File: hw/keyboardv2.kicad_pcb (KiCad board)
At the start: 2 copper layers, 145 x 45 mm, 40 parts, among them K1 CONN_4, K2 CONN_4, K3 CONN_4, K4 CONN_4, K5 CONN_4, K6 CONN_4, K7 CONN_4, K8 CONN_4, Q1 MOSFET_N, U1 TINYMEGA, U2 74HC595, U3 4051, U4 4051, U5 74HC595

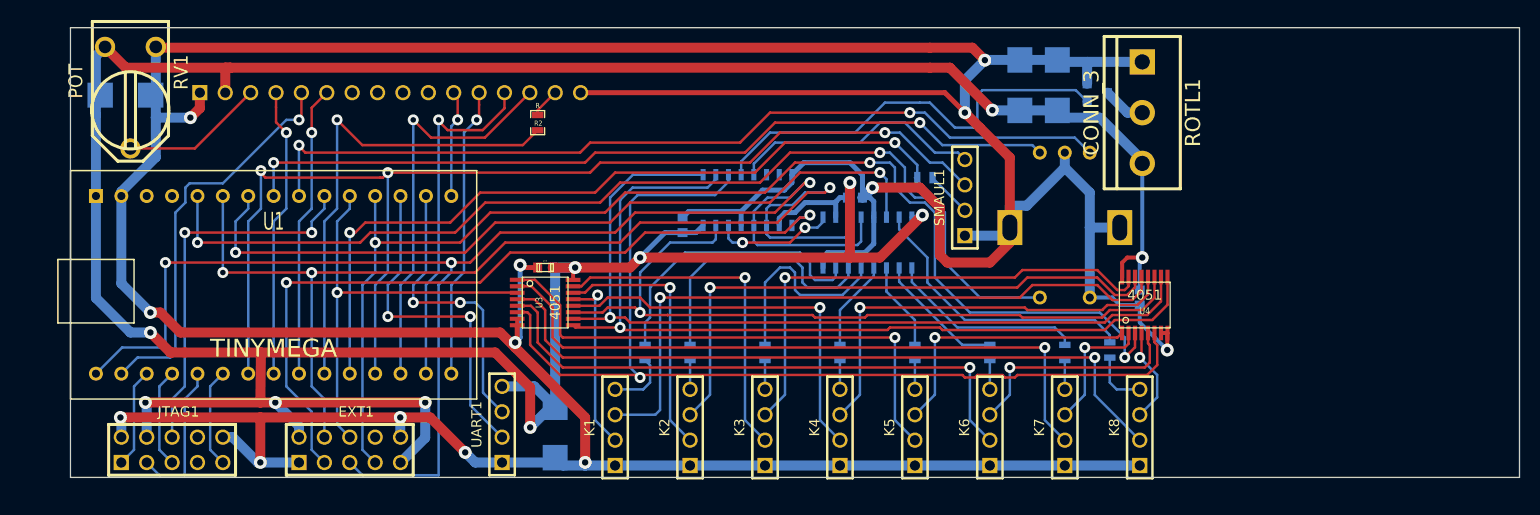
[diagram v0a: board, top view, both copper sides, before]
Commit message: Yeah, so I had the board reversed -.-   Once more with feeling.
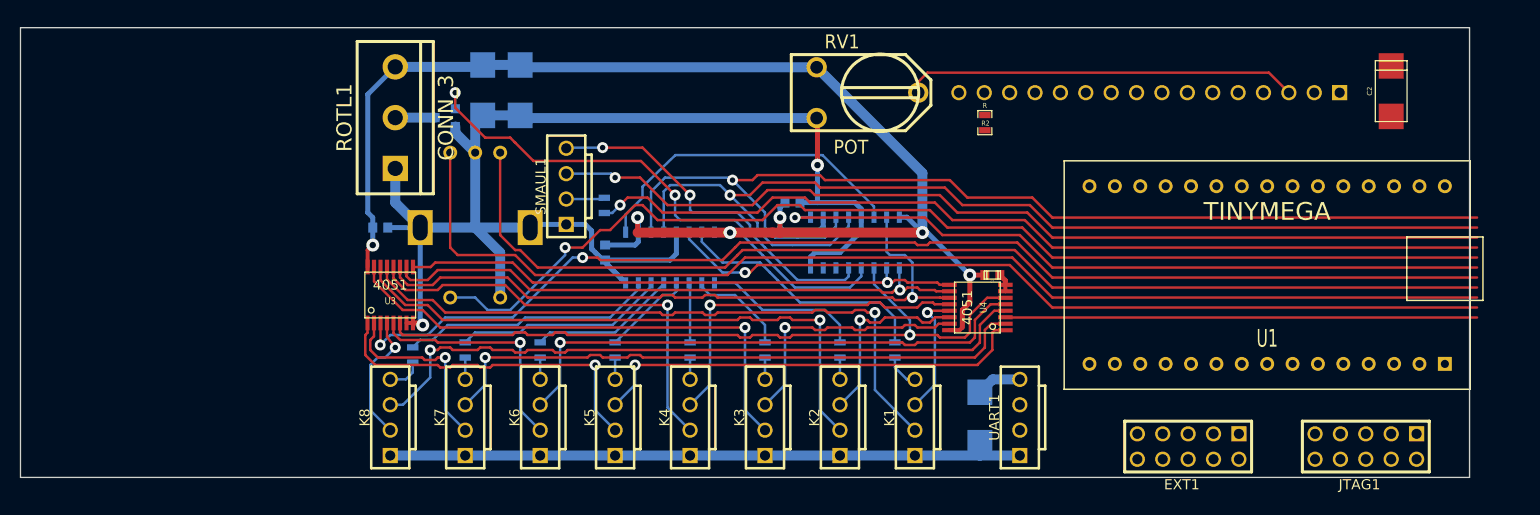
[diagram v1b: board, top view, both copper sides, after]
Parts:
- C2: moved to F.Cu
- K1, K2, K3, K4, K5, K6, K7, K8, SMAUL1, UART1: footprint PIN_ARRAY_4x1_BPAD -> PIN_ARRAY_4x1_KEYED_BPAD
- moved C2 126.7 mm to (212.2, 106.3), turned to 90 degrees
- moved JTAG1 119.5 mm to (209.6, 141.9), turned to 180 degrees
- moved U1 99.4 mm to (199.8, 124.8), turned to 180 degrees
- moved LCD1 95.0 mm to (207.0, 106.5), turned to 180 degrees
- moved EXT1 83.9 mm to (191.8, 141.9), turned to 180 degrees
- moved C6 76.3 mm to (111.0, 120.0), turned to 180 degrees
- moved K8 75.0 mm to (112.0, 139.0)
- moved ROTL1 74.8 mm to (112.5, 109.0), turned to 90 degrees
- moved RV1 73.8 mm to (159.8, 106.5), turned to 0 degrees
- moved R10 69.8 mm to (114.2, 132.8)
- moved Q1 65.3 mm to (117.5, 109.0), turned to 90 degrees
- moved K7 60.0 mm to (119.5, 139.0)
- moved R9 60.0 mm to (119.5, 132.2)
- moved S1 59.0 mm to (120.5, 120.0)
- moved C5 57.5 mm to (121.2, 106.2), turned to 90 degrees
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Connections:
- RV1 pad 1: GND -> VCC
- RV1 pad 3: VCC -> GND
- U5 pad 1: /Key Jacks/led6 -> /Key Jacks/led1
- U5 pad 15: /Key Jacks/led7 -> /Key Jacks/led0
- U5 pad 2: /Key Jacks/led5 -> /Key Jacks/led2
- U5 pad 3: /Key Jacks/led4 -> /Key Jacks/led3
- U5 pad 4: /Key Jacks/led3 -> /Key Jacks/led4
- U5 pad 5: /Key Jacks/led2 -> /Key Jacks/led5
- U5 pad 6: /Key Jacks/led1 -> /Key Jacks/led6
- U5 pad 7: /Key Jacks/led0 -> /Key Jacks/led7
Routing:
- net GND: track 491.5 -> 206.7 mm, vias 13 -> 2
- net VCC: track 350.7 -> 154.5 mm, vias 11 -> 6
- net /Key Jacks/KEY_SCIO: track 123.2 -> 47.2 mm, vias 3 -> 0
- net /Key Jacks/KEY_PWR: track 43.2 -> 118.1 mm, vias 1 -> 2
- net /Key Jacks/scio7: track 9.69 -> 68.9 mm
- net /Key Jacks/pwr7: track 72.1 -> 13.3 mm
- net /Key Jacks/scio0: track 67.0 -> 12.6 mm
- net /Key Jacks/pwr6: track 67.2 -> 19.0 mm
- net /LCD_LED: track 47.7 -> 0.00 mm, vias 1 -> 0
- net /Key Jacks/pwr0: track 18.1 -> 65.7 mm
- net /Key Jacks/scio6: track 13.2 -> 60.4 mm
- net /LCD_RW: track 40.2 -> 0.00 mm, vias 1 -> 0
- net /LCD_D3: track 40.2 -> 0.00 mm, vias 1 -> 0
- net /Key Jacks/scio1: track 58.6 -> 19.0 mm
- net /!RESET: track 37.9 -> 0.00 mm, vias 2 -> 0
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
